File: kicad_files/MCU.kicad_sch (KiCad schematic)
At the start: 24 parts, among them SW1 Boot, U1 RP2040, U2 W25Q128JVS, Y1 12MHz

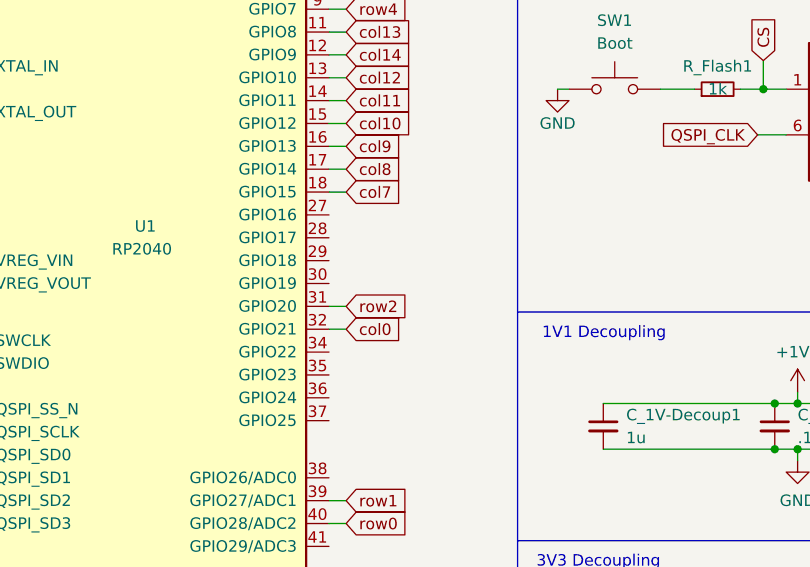
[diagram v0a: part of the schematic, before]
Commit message: double jst
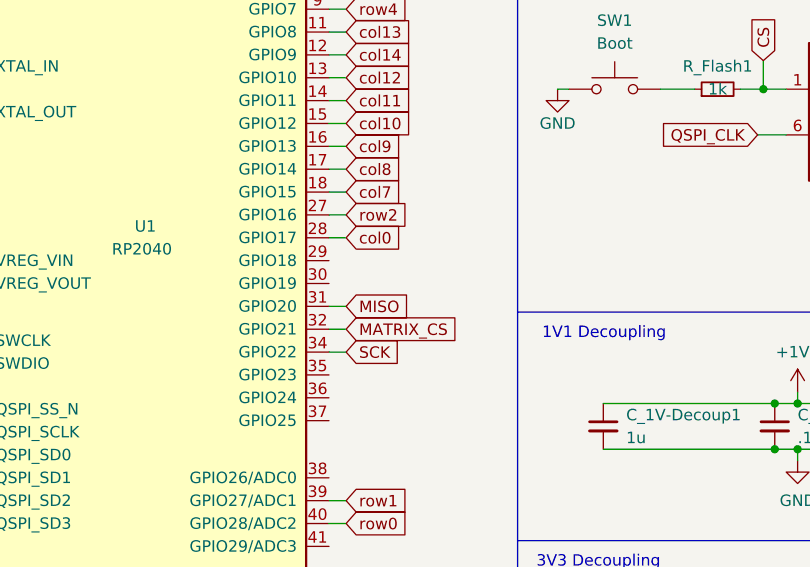
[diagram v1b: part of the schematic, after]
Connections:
- net col0: now also U1.28 (GPIO17); no longer U1.32 (GPIO21)
- net row2: now also U1.27 (GPIO16); no longer U1.31 (GPIO20)
- net SCK: now reaches U1.34 (GPIO22)
- new net MATRIX_CS: U1.32 (GPIO21)
- new net MISO: U1.31 (GPIO20)
